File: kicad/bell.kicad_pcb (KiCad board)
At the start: 2 copper layers, 39 parts, among them IC1 ATTINY13A-SS, P1 CONN_2, P2 CONN_3X2, Q1 BD137, Q2 BC556, Q3 BC556, SW1 SWITCH_INV, T1 TRANSFO_4, U1 LM7805CT

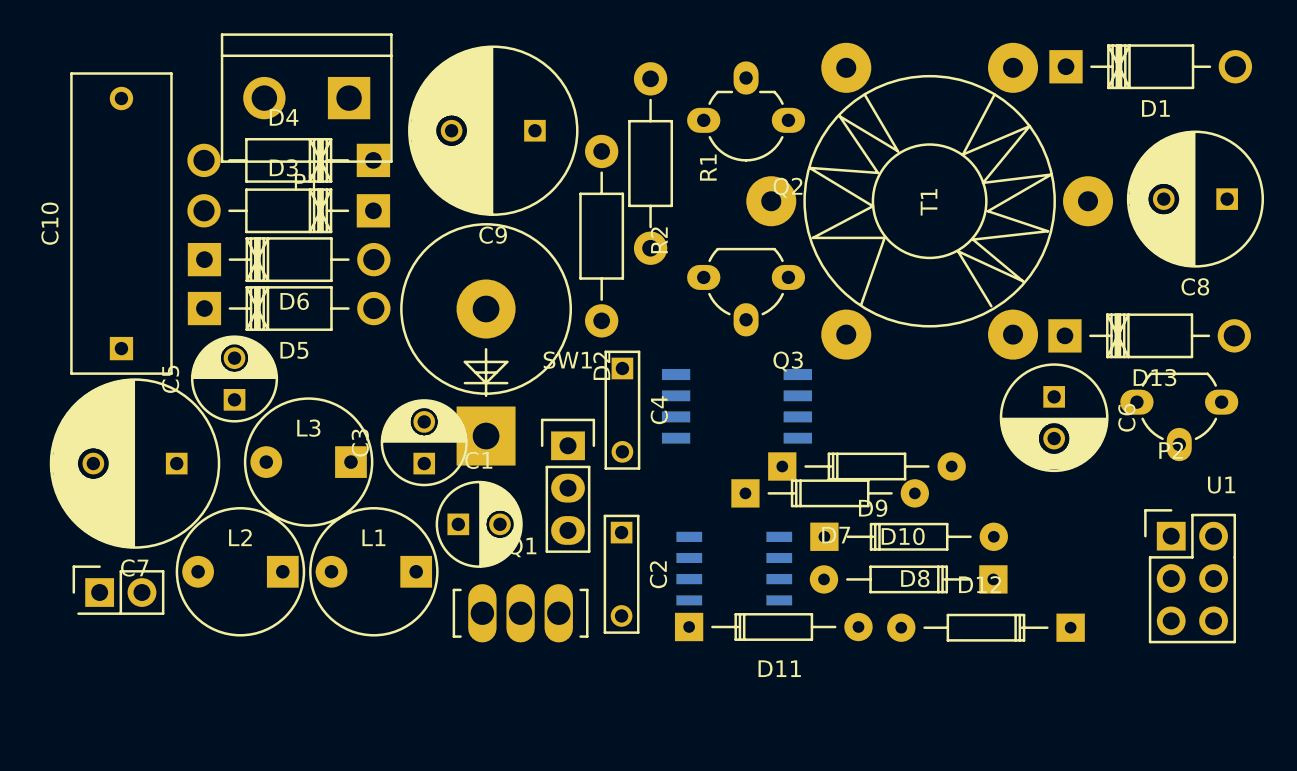
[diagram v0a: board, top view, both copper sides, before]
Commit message: Board
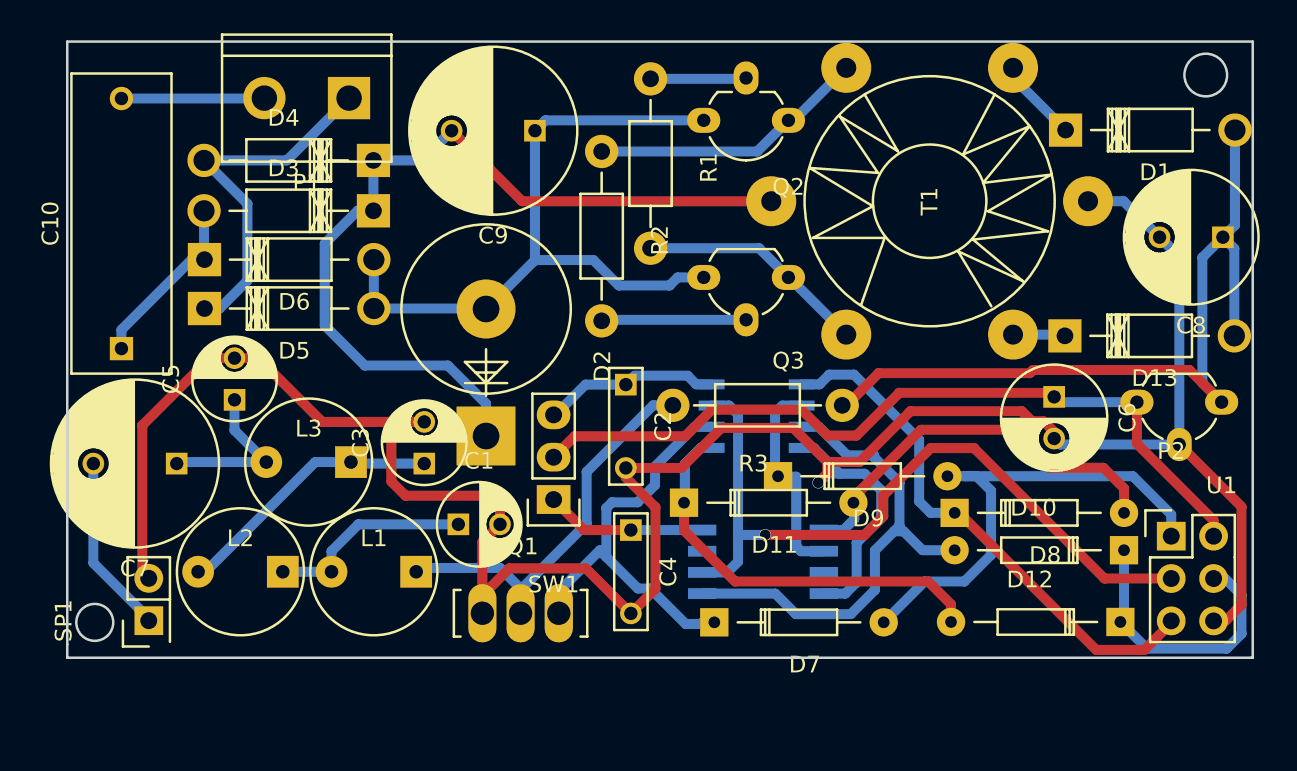
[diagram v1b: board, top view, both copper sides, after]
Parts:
- added R3: R, Resistors_ThroughHole:Resistor_Horizontal_RM10mm, F.Cu at (101.5, 41.9)
- moved C4 9.70 mm to (88.8, 49.4)
- moved DD1 9.45 mm to (96.8, 51.3)
- moved IC1 9.24 mm to (96.4, 42.6)
- moved C2 8.88 mm to (88.5, 40.7)
- moved D10 8.03 mm to (118.4, 50.6)
- moved D7 7.96 mm to (93.9, 55.0)
- moved D8 7.94 mm to (108.3, 48.4)
- moved D11 7.46 mm to (92.0, 47.8)
- moved D1 3.80 mm to (114.9, 25.4)
- moved SP1 3.40 mm to (59.9, 54.9), turned to 90 degrees
- moved SW1 3.34 mm to (84.2, 47.6), turned to 180 degrees
- moved D12 3.00 mm to (118.2, 54.9)
- moved C8 2.30 mm to (124.4, 31.9)
- moved D9 0.64 mm to (97.7, 46.2)
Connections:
- net Net-(C8-Pad1) renamed +5V
- Q1 pad 1: Net-(L1-Pad1) -> GNDPWR
- Q1 pad 2: (no net) -> Net-(L1-Pad1)
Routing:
- net GNDPWR: track 0.00 -> 157.6 mm, vias 0 -> 1
- net Net-(C9-Pad2): track 0.00 -> 51.6 mm
- net +5V: track 0.00 -> 48.3 mm
- net VDD: track 0.00 -> 47.9 mm
- net Net-(DD1-Pad6): track 0.00 -> 45.4 mm, vias 0 -> 1
- net Net-(C9-Pad1): track 0.00 -> 43.2 mm
- net Net-(D8-Pad1): track 0.00 -> 32.5 mm
- net Net-(D10-Pad2): track 0.00 -> 29.9 mm
- net Net-(D7-Pad2): track 0.00 -> 29.6 mm
- net Net-(D7-Pad1): track 0.00 -> 26.3 mm
- net Net-(L1-Pad1): track 0.00 -> 25.3 mm
- net Net-(D11-Pad2): track 0.00 -> 24.9 mm
- net Net-(D11-Pad1): track 0.00 -> 24.7 mm
- net Net-(D4-Pad2): track 0.00 -> 21.8 mm
- net Net-(D10-Pad1): track 0.00 -> 17.3 mm
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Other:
- board outline added: 71.1 x 37 mm

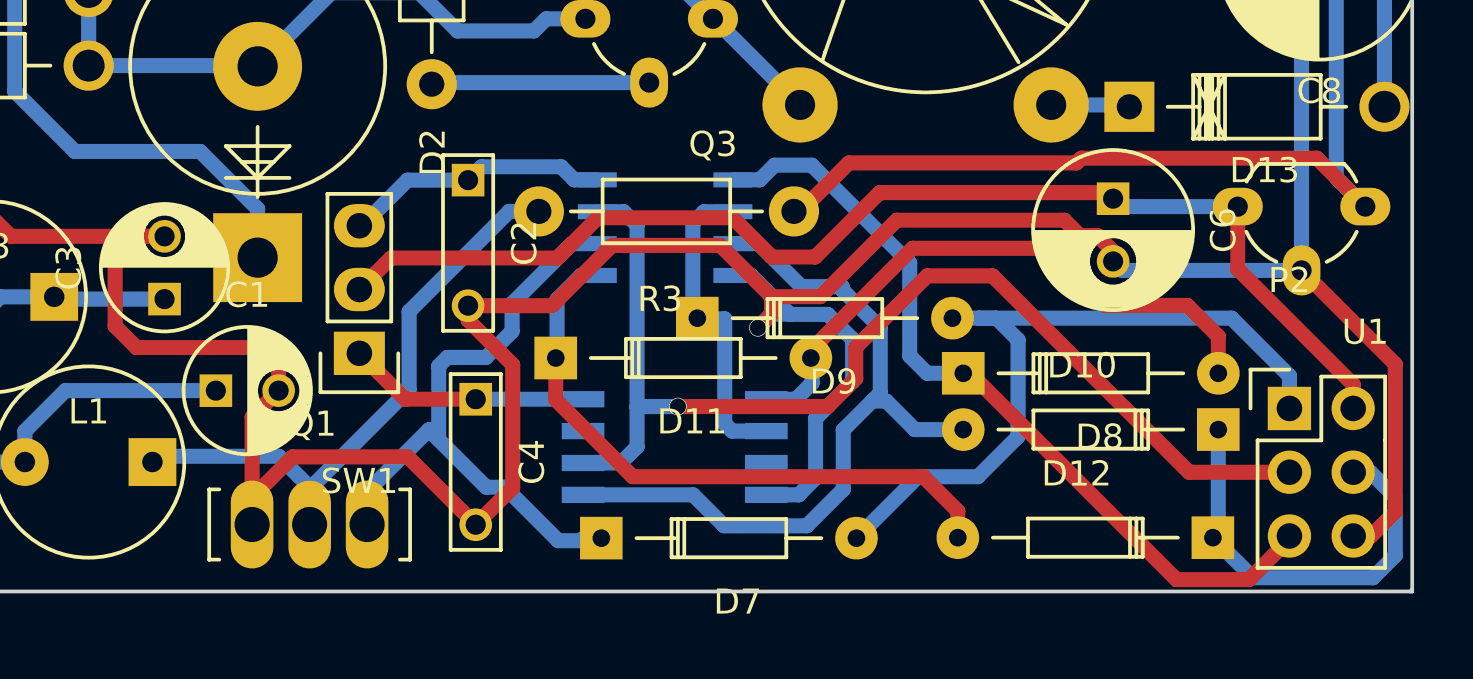
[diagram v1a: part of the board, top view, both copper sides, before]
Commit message: New
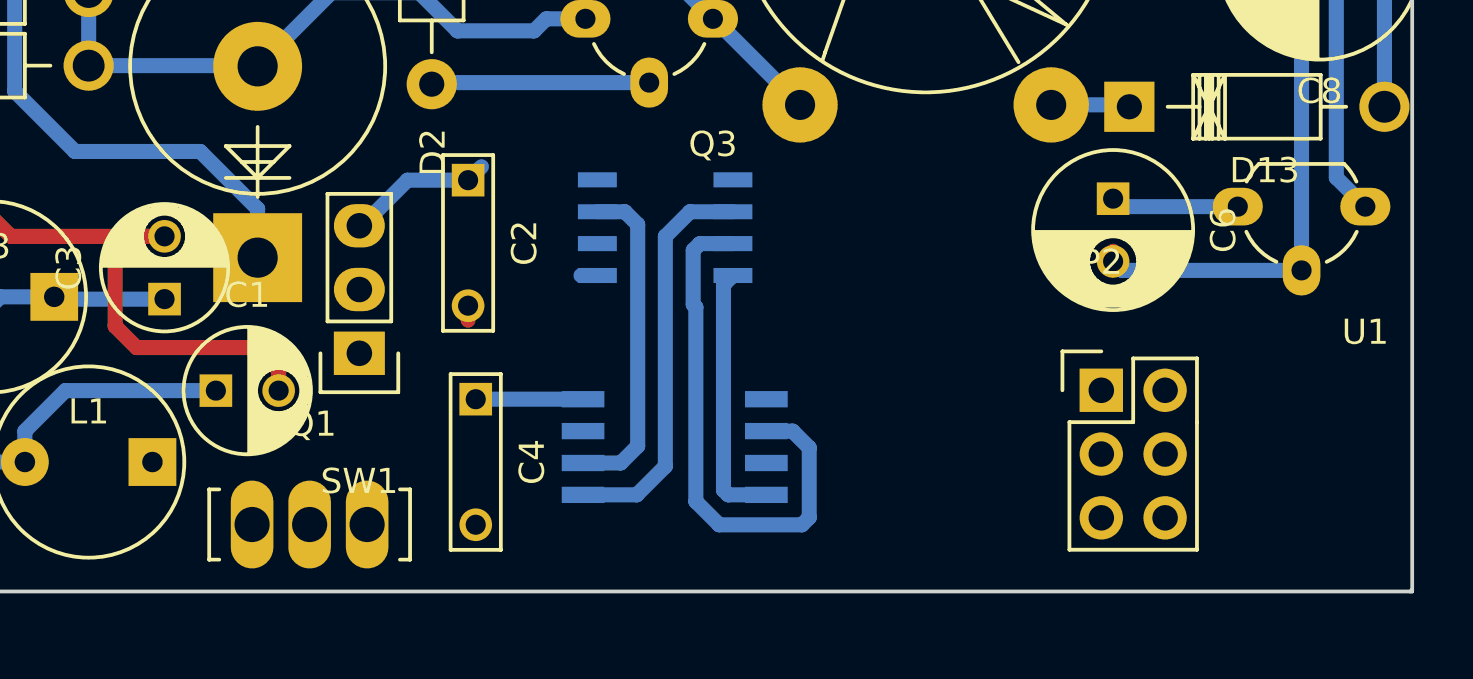
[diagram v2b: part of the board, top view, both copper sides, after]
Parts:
- removed D10, D11, D12, D7, D8, D9: DIODE, Diodes_ThroughHole:Diode_DO-35_SOD27_Horizontal_RM10
- removed R3: R, Resistors_ThroughHole:Resistor_Horizontal_RM10mm
- moved P2 7.53 mm to (113.8, 49.1)
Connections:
- DD1 pad 1: Net-(D11-Pad2) -> Net-(DD1-Pad1)
- DD1 pad 2: Net-(D9-Pad1) -> Net-(DD1-Pad2)
- DD1 pad 5: Net-(D10-Pad2) -> Net-(DD1-Pad5)
- IC1 pad 1: Net-(D8-Pad1) -> (no net)
- IC1 pad 2: Net-(D9-Pad1) -> Net-(DD1-Pad5)
- IC1 pad 3: Net-(D10-Pad2) -> Net-(DD1-Pad2)
- IC1 pad 5: Net-(D11-Pad1) -> Net-(IC1-Pad5)
- IC1 pad 6: Net-(D7-Pad1) -> Net-(DD1-Pad1)
- P2 pad 1: Net-(D7-Pad2) -> Net-(DD1-Pad2)
- P2 pad 4: Net-(D10-Pad1) -> Net-(DD1-Pad5)
- P2 pad 5: Net-(D8-Pad1) -> Net-(DD1-Pad1)
- Q1 pad 1: GNDPWR -> Net-(L1-Pad1)
- Q1 pad 2: Net-(L1-Pad1) -> (no net)
- Q1 pad 3: Net-(D7-Pad1) -> Net-(IC1-Pad5)
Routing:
- net GNDPWR: track 157.6 -> 81.3 mm, vias 1 -> 0
- net VDD: track 47.9 -> 5.10 mm
- net Net-(D8-Pad1): track 32.5 -> 0.00 mm
- net Net-(DD1-Pad6): track 45.4 -> 13.1 mm, vias 1 -> 0
- net Net-(D10-Pad2): track 29.9 -> 0.00 mm
- net Net-(D7-Pad2): track 29.6 -> 0.00 mm
- net Net-(D7-Pad1): track 26.3 -> 0.00 mm
- net Net-(D11-Pad2): track 24.9 -> 0.00 mm
- net Net-(D11-Pad1): track 24.7 -> 0.00 mm
- net +5V: track 48.3 -> 23.8 mm
- net Net-(L1-Pad1): track 25.3 -> 1.40 mm
- net Net-(DD1-Pad2): track 0.00 -> 21.5 mm
- net Net-(D10-Pad1): track 17.3 -> 0.00 mm
- net Net-(DD1-Pad5): track 0.00 -> 16.0 mm
- net Net-(D9-Pad1): track 12.8 -> 0.00 mm
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
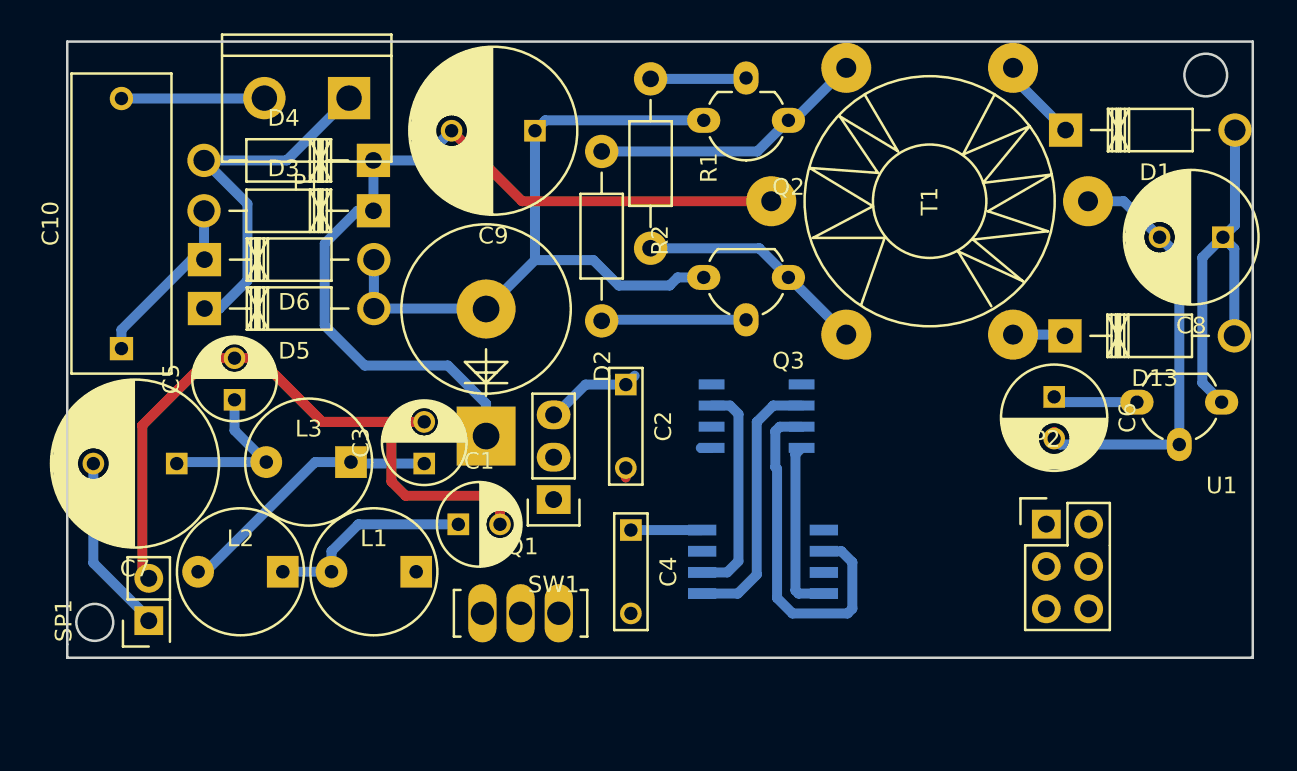
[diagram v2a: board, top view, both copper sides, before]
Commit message: Fix
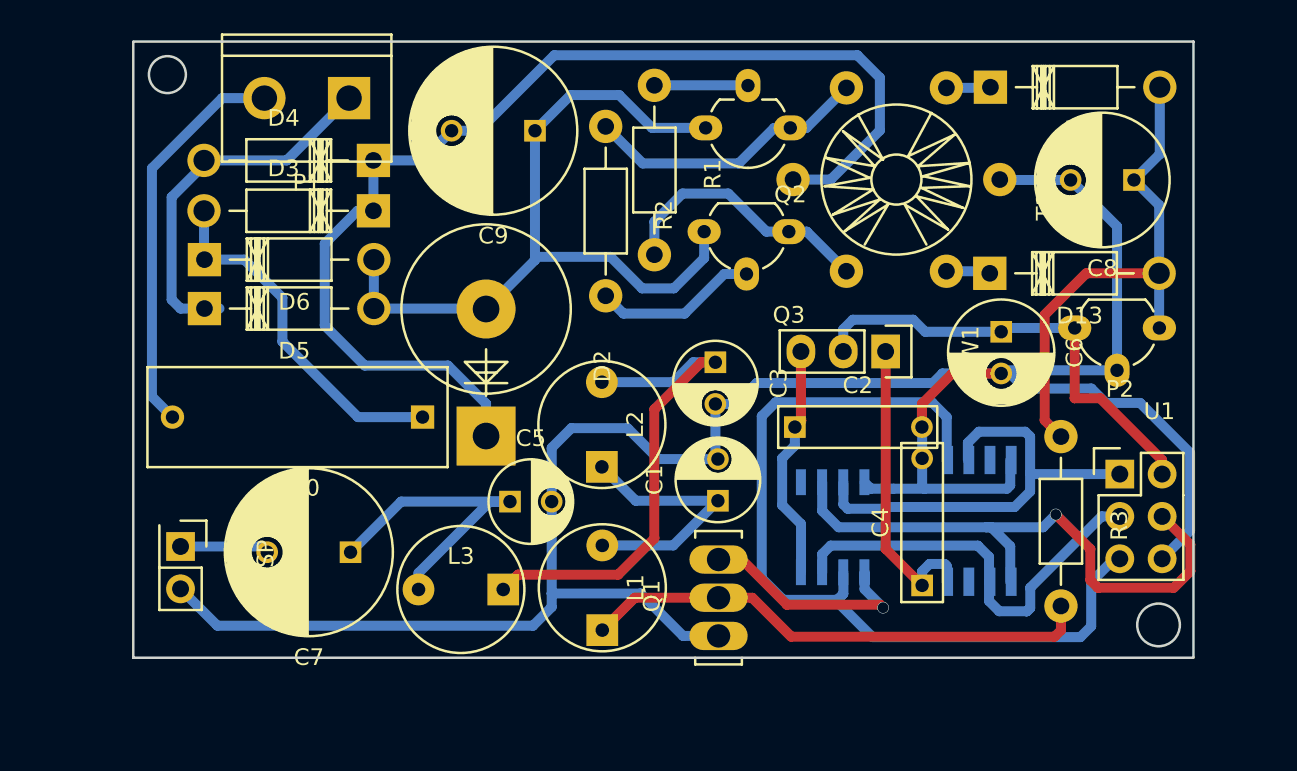
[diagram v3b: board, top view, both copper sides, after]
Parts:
- removed IC1: ATTINY13A-SS, Housings_SOIC:SOIC-8_3.9x4.9mm_Pitch1.27mm
- added DD2: w25q64fvssig, Housings_SOIC:SOIJ-8_5.3x5.3mm_Pitch1.27mm, B.Cu at (109.8, 48.9)
- added R3: 5.1, Resistors_ThroughHole:Resistor_Horizontal_RM10mm, F.Cu at (114.6, 43.8)
- C1: value CP1 -> 2.2
- C10: value C -> 2.2
- C2, C4: value C -> 0.1; footprint Capacitors_ThroughHole:C_Rect_L7_W2_P5 -> cymometer:C_Rect_L10_W2.5_P5
- C3, C5: value CP1 -> 1.0
- C6: value CP1 -> 10.0
- C7: value CP1 -> 100.0
- C8: value CP1 -> 470.0
- C9: value CP1 -> 22.0
- D2: value ZENER -> Д816Г
- D3, D4, D5, D6: value DIODE -> 1N4007
- DD1: value w25q64fvssig -> ATTINY13A-SS; footprint Housings_SOIC:SOIJ-8_5.3x5.3mm_Pitch1.27mm -> Housings_SOIC:SOIC-8_3.9x4.9mm_Pitch1.27mm
- L1: value INDUCTOR -> 150 uH
- L2, L3: value INDUCTOR -> 20 uH
- Q2, Q3: value BC556 -> КТ313
- R1, R2: value R -> 5.1 k
- T1: footprint Choke_Toroid_ThroughHole:Transformer_Toroid_Tapped_Horizontal_Diameter14mm_Amidon-T50 -> Choke_Toroid_ThroughHole:Transformer_Toroid_Tapped_horizontal_Diameter9mm_Amidon-T30
- moved L2 23.4 mm to (87.1, 43.1), turned to 90 degrees
- moved SW1 21.8 mm to (104.1, 38.7), turned to 270 degrees
- moved C10 18.5 mm to (76.4, 42.6), turned to 180 degrees
- moved C3 18.5 mm to (93.9, 39.4), turned to 270 degrees
- moved C5 17.6 mm to (81.6, 47.7), turned to 0 degrees
- moved C4 17.5 mm to (106.3, 48.9), turned to 90 degrees
- moved C1 15.6 mm to (94.1, 47.7), turned to 90 degrees
- moved C2 14.2 mm to (102.5, 43.2), turned to 0 degrees
- moved L1 13.7 mm to (87.1, 52.9), turned to 90 degrees
- moved Q1 11.9 mm to (94.1, 53.5), turned to 90 degrees
- moved L3 11.9 mm to (78.7, 53.0)
- moved C7 11.7 mm to (72.0, 50.7)
- moved C8 6.34 mm to (119.0, 28.4)
- moved D13 5.87 mm to (110.4, 34.0)
- moved U1 5.81 mm to (120.5, 37.3)
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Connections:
- DD1 pad 1: Net-(DD1-Pad1) -> (no net)
- DD1 pad 3: (no net) -> Net-(DD1-Pad3)
- DD1 pad 7: (no net) -> Net-(DD1-Pad7)
- DD1 pad 8: Net-(C4-Pad1) -> Net-(C2-Pad1)
- P2 pad 1: Net-(DD1-Pad2) -> Net-(DD1-Pad3)
- P2 pad 3: Net-(DD1-Pad6) -> Net-(DD1-Pad7)
- P2 pad 4: Net-(DD1-Pad5) -> Net-(DD1-Pad2)
- P2 pad 5: Net-(DD1-Pad1) -> Net-(DD1-Pad6)
- Q1 pad 1: Net-(L1-Pad1) -> GNDPWR
- Q1 pad 2: (no net) -> Net-(L1-Pad1)
- Q1 pad 3: Net-(IC1-Pad5) -> Net-(DD1-Pad5)
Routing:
- net GNDPWR: track 81.3 -> 142.9 mm
- net Net-(DD1-Pad6): track 13.1 -> 52.5 mm
- net Net-(L1-Pad1): track 1.40 -> 30.9 mm
- net Net-(DD1-Pad3): track 0.00 -> 26.6 mm
- net Net-(DD1-Pad7): track 0.00 -> 25.0 mm
- net VDD: track 5.10 -> 27.7 mm
- net Net-(C9-Pad2): track 51.6 -> 68.4 mm
- net Net-(C10-Pad2): track 8.58 -> 24.0 mm
- net Net-(DD1-Pad2): track 21.5 -> 35.9 mm, vias 0 -> 1
- net Net-(C4-Pad1): track 4.27 -> 18.4 mm
- net Net-(C3-Pad1): track 16.3 -> 30.2 mm
- net Net-(C10-Pad1): track 10.8 -> 21.5 mm
- net Net-(C5-Pad1): track 9.93 -> 19.1 mm
- net Net-(C2-Pad1): track 5.68 -> 14.8 mm
- net +5V: track 23.8 -> 31.8 mm
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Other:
- board size 71.1 x 37 mm -> 63.6 x 37 mm
